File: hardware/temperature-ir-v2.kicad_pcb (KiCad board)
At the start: 2 copper layers, 20 x 25 mm, 24 parts, among them P1 CON-SENSOR2, P2 DEBUG, P3 BOOT, U1 XMC110024, U2 MLX90614, U4 DRILL, U5 DRILL, U6 DRILL, U7 DRILL

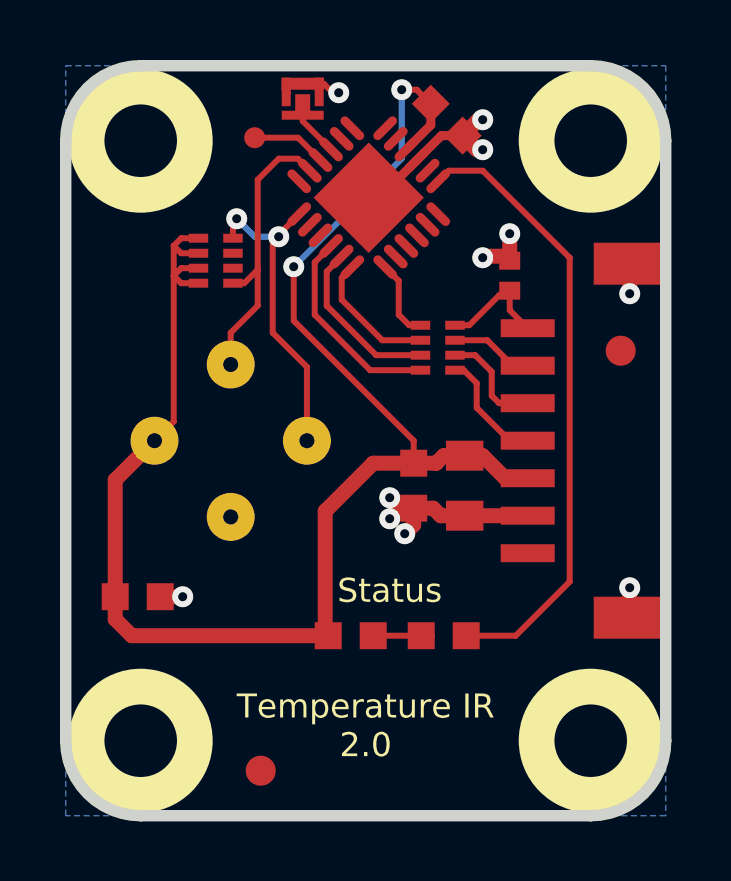
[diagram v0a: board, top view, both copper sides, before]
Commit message: move to new kicad version
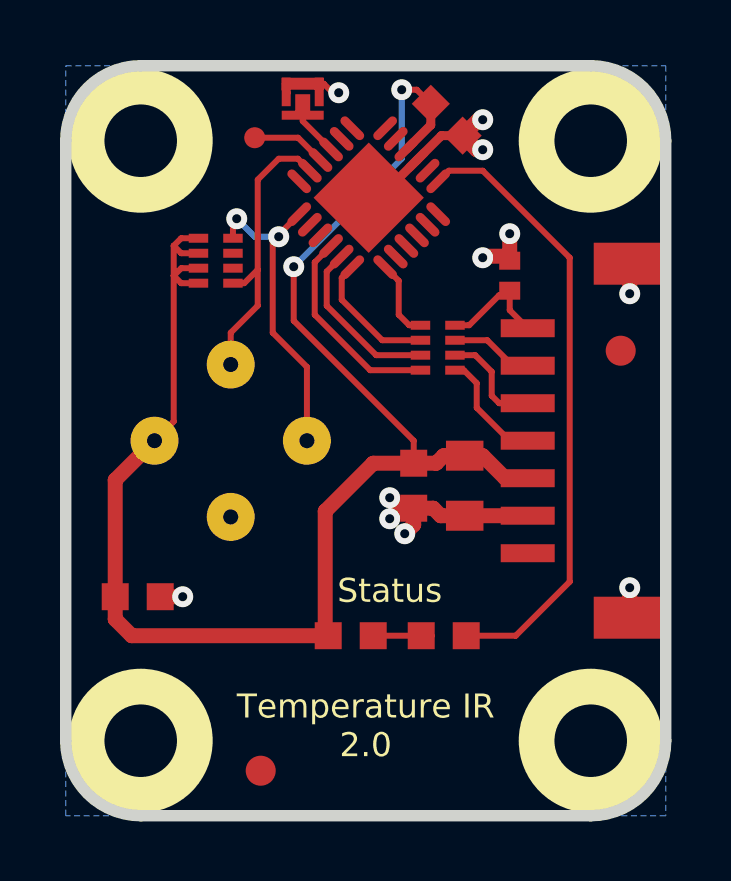
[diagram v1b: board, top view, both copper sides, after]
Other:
- net class Default removed
